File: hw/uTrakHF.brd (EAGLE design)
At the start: 12.7 x 47.9 mm, 60 parts, among them Q1 PMDPB58UPE, U1 MSP430FR5738, U2 SI5351C, U3 PL133-27, U4 SPV1050

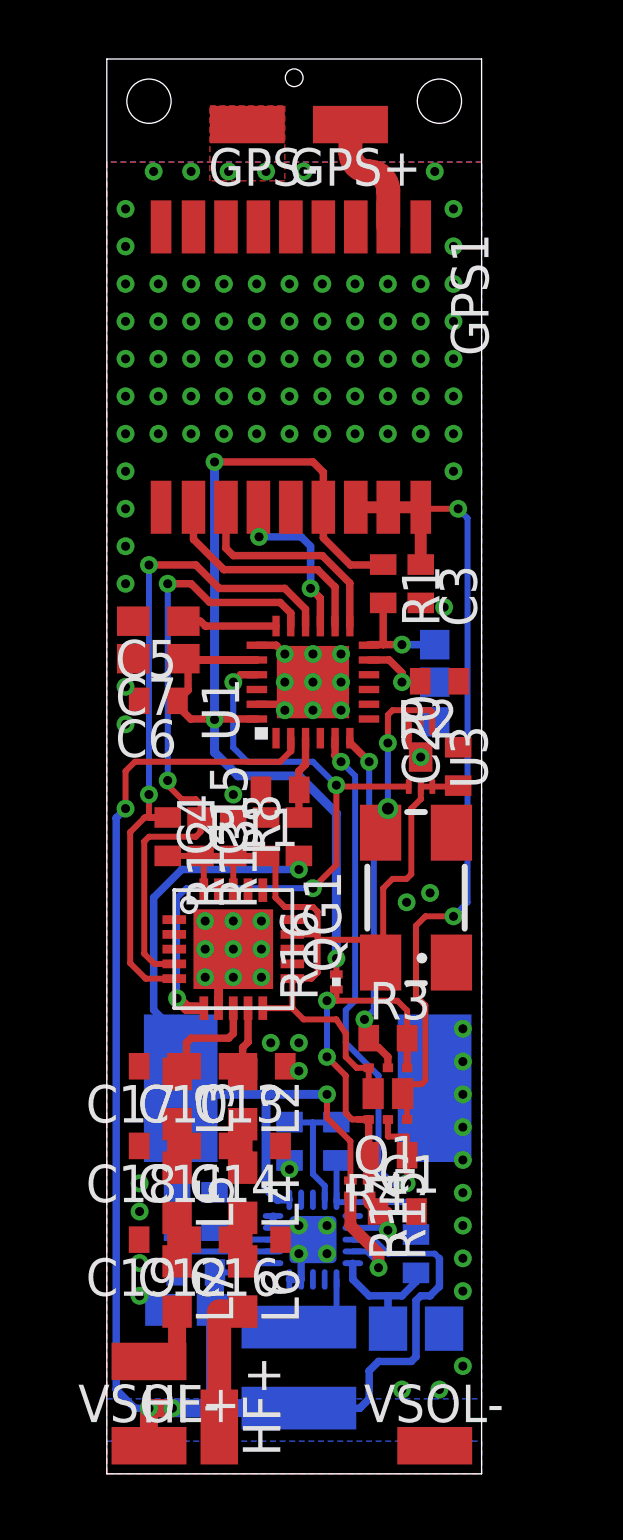
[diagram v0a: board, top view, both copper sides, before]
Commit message: update hardware design documentation
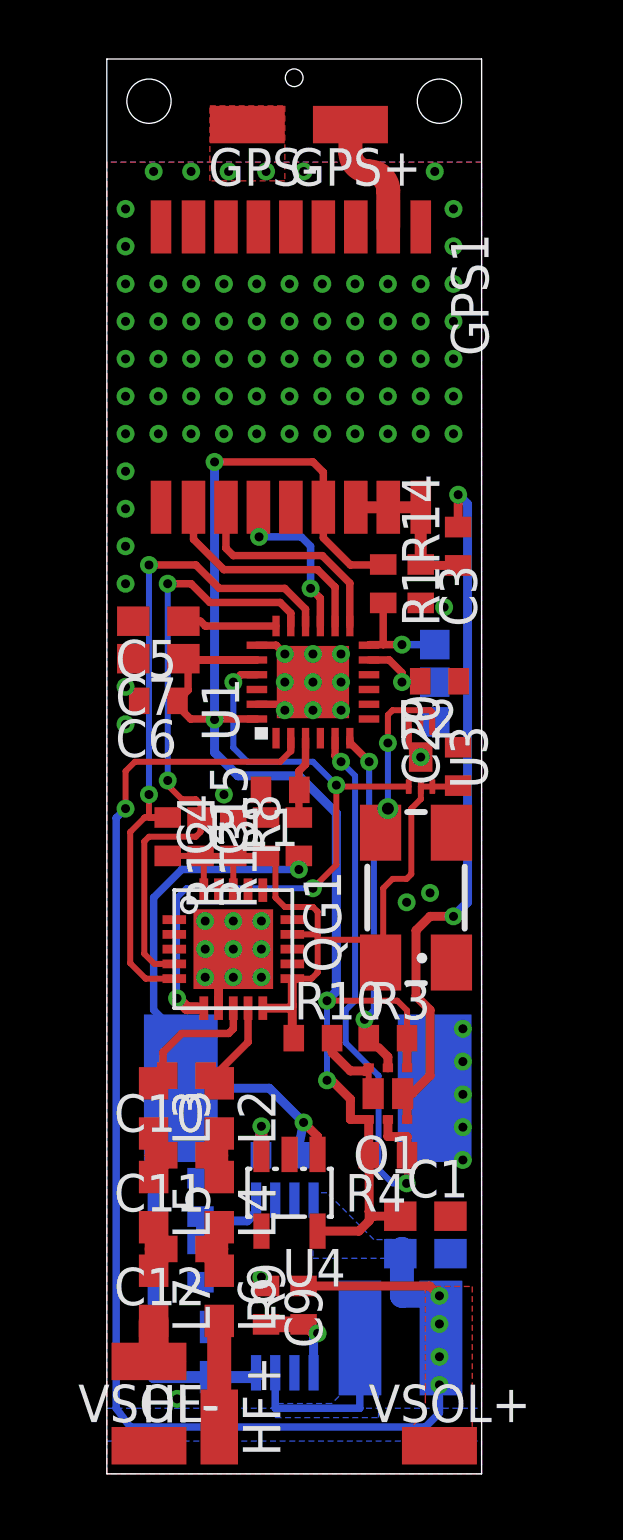
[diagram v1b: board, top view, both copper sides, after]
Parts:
- removed C13, C17: DNP (320p), rcl:C0402
- removed C14, C18: DNP (400p), rcl:C0402
- removed C16, C19: DNP (200p), rcl:C0402
- removed R15, R16: 0, rcl:R0201
- added U5: SPV1040, spv1040:TSSOP8
- C1: value 100n -> 1u; device rcl:C0402 -> rcl:C0603
- C2: value 47u -> 10u; device rcl:C0805 -> rcl:C0603
- C8: value 4u7 -> 10u; device rcl:C0603K -> rcl:C0603
- C9: value 10n -> 100n
- L1: value 22u -> 10u
- R10: value 8M2 -> 4R7
- R14: value 0 -> 4R7; device rcl:R0201 -> rcl:R0402
- R5: value 6M8 -> 1M
- R6: value 1M5 -> 100k
- R7: value 2M7 -> 384k
- R9: value 3M3 -> 1k
- U4: value SPV1050 -> MIC5304; device SPV1050:SPV1050 -> v-reg-micrel:SOT23-5
- moved R14 22.1 mm to (11.9, 31.4), turned to 90 degrees
- moved VSOL+ 9.84 mm to (11.3, 0.95)
- moved VSOL- 9.68 mm to (1.43, 0.95)
- moved R5 7.55 mm to (3.17, 9.37)
- moved R10 7.46 mm to (6.99, 14.8), flipped to the top, turned to 0 degrees
- moved R7 5.11 mm to (3.17, 7.14), turned to 90 degrees
- moved R9 3.82 mm to (6.67, 5.71), flipped to the top, turned to 90 degrees
- moved C9 3.62 mm to (5.40, 5.71), flipped to the top, turned to 270 degrees
- moved L1 3.62 mm to (10.0, 4.60), turned to 180 degrees
- moved C2 2.56 mm to (10.8, 7.46)
- moved R6 1.96 mm to (5.87, 10.8), turned to 180 degrees
- moved U4 1.77 mm to (6.19, 9.53), flipped to the top
- moved C8 1.72 mm to (3.65, 4.13), turned to 90 degrees
- moved C1 0.97 mm to (10.8, 8.73)
- moved C11 0.85 mm to (2.70, 10.8)
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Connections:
- removed net N$10: L1.2, U4.16
- removed net N$13: R10.1, R9.2, U4.2
- removed net N$14: C9.1, U4.3
- removed net PGND: U4.18
- new net N$1: Q1.3, Q1.8, R10.2
- new net N$20: R5.1, R7.2, U5.5
- new net VBAT: C8.1, R5.2, R6.2, R8.1, U4.1, U5.4, UC1.2
- net +3V3: now also U4.5; no longer R15.1, R15.2, R16.1, R16.2, U4.12
- net +3V3_GPS: now also R14.1; no longer Q1.6, Q1.7
- net +3V3_SI: now also R10.1; no longer Q1.3, Q1.8
- net C33: no longer C13.2
- net GND: now also C9.1, R7.1, U4.2, U5.2, U5.6, U5.7; no longer C13.1, C14.1, C16.1, C17.2, C18.2, C19.2, C9.2, R10.2, R7.2, U4.19, U4.20, U4.4, U4.5, U4.EXP
- net N$12: no longer C17.1
- net N$15: no longer C18.1
- net N$16: no longer C19.1
- net N$3: no longer C14.2
- net N$4: now also Q1.6, Q1.7; no longer R14.1, R8.1, U4.14, U4.6, UC1.2
- net N$5: no longer C16.2
- net N$6: now also U4.3; no longer R5.2, U4.10
- net N$7: now also L1.1, U5.3; no longer R6.2, R7.1, U4.9
- net N$8: now also C9.2, R9.1, U5.1; no longer C2.1, R5.1, U4.15
- net VSOL_IN: now also C2.1, L1.2, R9.2, U5.8; no longer C8.1, L1.1, R9.1, U4.1, U4.13
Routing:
- net VBAT: track 0.00 -> 38.6 mm, vias 0 -> 2
- net +3V3_GPS: track 28.9 -> 5.49 mm, vias 2 -> 0
- net VSOL_IN: track 57.0 -> 48.7 mm, vias 3 -> 5
- net N$4: track 30.0 -> 24.5 mm, vias 3 -> 2
- net N$13: track 4.71 -> 0.00 mm
- net +3V3_SI: track 32.3 -> 27.9 mm
- net N$1: track 0.00 -> 3.75 mm
- net N$20: track 0.00 -> 3.39 mm
- net GND: track 8.86 -> 5.47 mm, vias 119 -> 101
- net N$6: track 5.02 -> 1.94 mm, vias 0 -> 1
- net N$10: track 2.55 -> 0.00 mm
- net N$14: track 2.12 -> 0.00 mm
- net N$7: track 4.39 -> 6.45 mm
- net N$8: track 4.53 -> 3.27 mm, vias 0 -> 1
- net HF+: track 4.94 -> 3.83 mm
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- added copper zone on layer 16, net N$7
- added copper zone on layer 1, net VSOL_IN
- added copper zone on layer 16, net VSOL_IN
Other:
- board text added: "uTrakHF GPS Tracker v1.1 High altitude balloon payload www.loetlabor-jena.de"
- board text removed: "uTrakHF GPS Tracker v1.0 High altitude balloon payload www.loetlabor-jena.de"
